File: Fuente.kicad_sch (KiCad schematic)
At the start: 0 parts

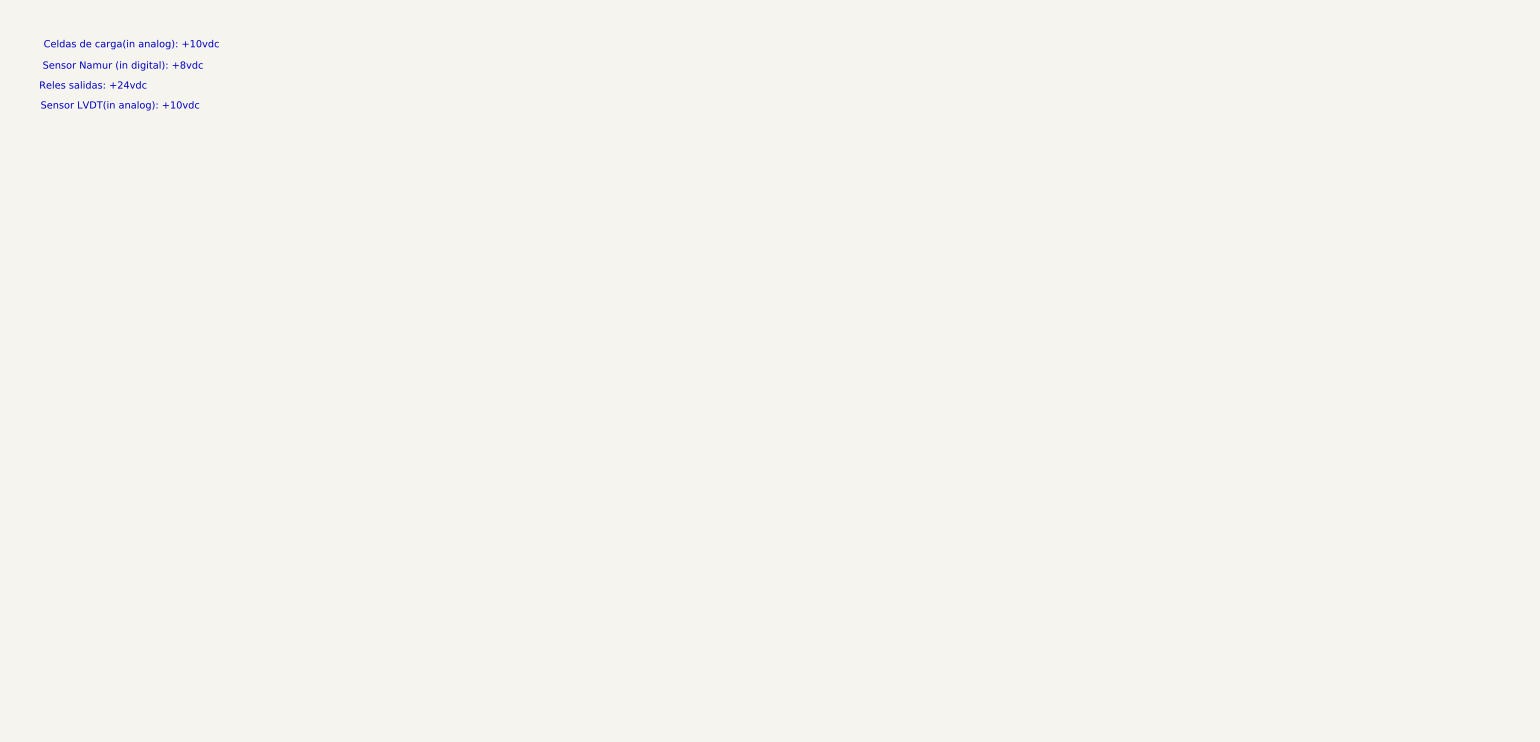
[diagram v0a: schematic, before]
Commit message: Avance
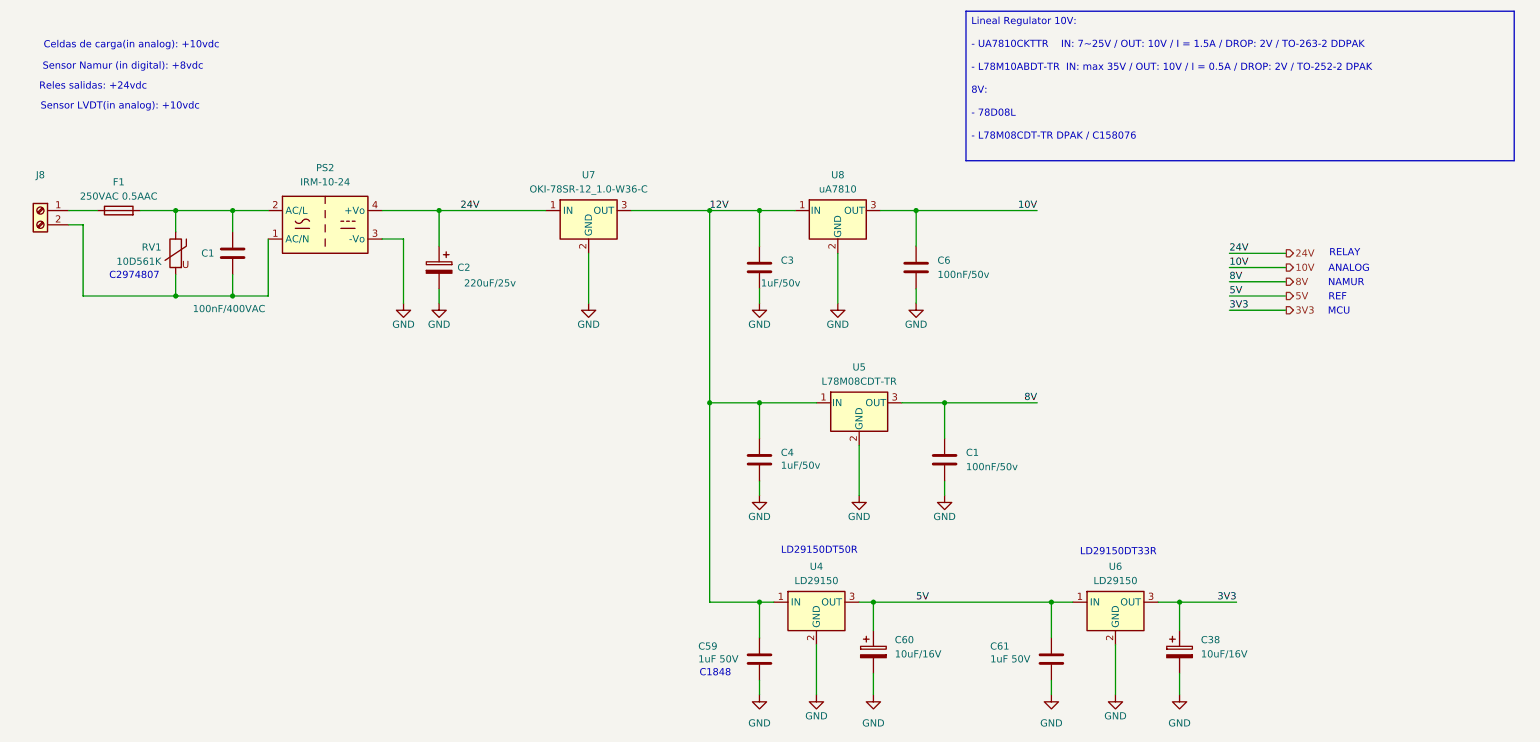
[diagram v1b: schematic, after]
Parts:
- added C1: 100nF/400VAC, Capacitor_THT:C_Disc_D10.5mm_W5.0mm_P7.50mm, symbol Device:C
- added C1, C6: 100nF/50v, 1-Capacitor:C_0805_2012Metric, symbol Device:C
- added C2: 220uF/25v, Capacitor_THT:CP_Radial_D8.0mm_P3.50mm, symbol Device:C_Polarized
- added C3, C4: 1uF/50v, 1-Capacitor:C_1206_3216Metric, symbol 1-Capacitor:C_1206
- added C38, C60: 10uF/16V, Capacitor_THT:CP_Radial_D5.0mm_P2.50mm, symbol Device:C_Polarized
- added C59, C61: 1uF 50V, 1-Capacitor:C_1206_3216Metric, symbol 1-Capacitor:C_0805
- added F1: 250VAC 0.5AAC, Fuse:Fuseholder_TR5_Littelfuse_No560_No460, symbol Device:Fuse
- added J8: Screw_Terminal_01x02, 1-Terminal-Block:DG126_5.0_02P, symbol 1-Terminal-Block:DG126_5.0_02P
- added PS2: IRM-10-24, Converter_ACDC:Converter_ACDC_MeanWell_IRM-10-xx_THT, symbol Converter_ACDC:IRM-10-24
- added RV1: 10D561K, Varistor:RV_Disc_D12mm_W3.9mm_P7.5mm, symbol Device:Varistor
- added U4, U6: LD29150, Package_TO_SOT_SMD:TO-252-2, symbol LIB_SCH_CONTR:LD29150
- added U5: L78M08CDT-TR, Package_TO_SOT_SMD:TO-252-2, symbol Regulator_Linear:uA7810
- added U7: OKI-78SR-12_1.0-W36-C, Converter_DCDC:Converter_DCDC_Murata_OKI-78SR_Vertical, symbol Converter_DCDC:OKI-78SR-12_1.0-W36-C
- added U8: uA7810, Package_TO_SOT_SMD:TO-263-3_TabPin2, symbol Regulator_Linear:uA7810
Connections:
- new net: F1.1, J8.1 (Pin_1)
- new net: C1.1, F1.2, PS2.2 (AC/L), RV1.1
- new net: C1.2, J8.2 (Pin_2), PS2.1 (AC/N), RV1.2
- new net 10V: C6.1, U8.3 (OUT)
- new net 12V: C3.1, C4.1, C59.1, U4.1 (IN), U5.1 (IN), U7.3 (OUT), U8.1 (IN)
- new net 24V: C2.1, PS2.4 (+Vo), U7.1 (IN)
- new net 3V3: C38.1, U6.3 (OUT)
- new net 5V: C60.1, C61.1, U4.3 (OUT), U6.1 (IN)
- new net 8V: C1.1, U5.3 (OUT)
- new net GND: C1.2, C2.2, C3.2, C38.2, C4.2, C59.2, C6.2, C60.2, C61.2, PS2.3 (-Vo), U4.2 (GND), U5.2 (GND), U6.2 (GND), U7.2 (GND), U8.2 (GND)
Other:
- note added: "ANALOG"
- note added: "C1848"
- note added: "C2974807"
- note added: "LD29150DT33R"
- note added: "LD29150DT50R"
- note added: "MCU"
- note added: "NAMUR"
- note added: "REF"
- note added: "RELAY"
